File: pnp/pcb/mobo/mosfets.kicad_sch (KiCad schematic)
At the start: 0 parts

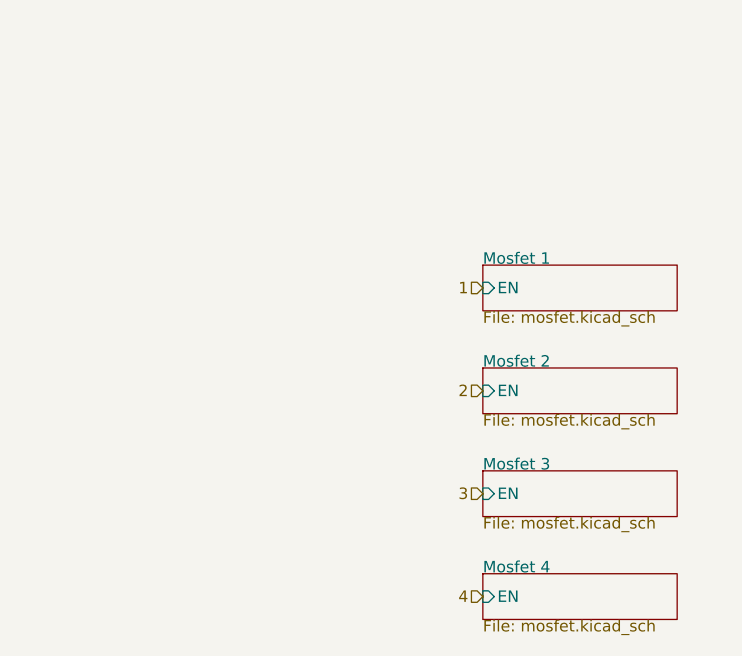
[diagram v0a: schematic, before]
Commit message: All pages checked
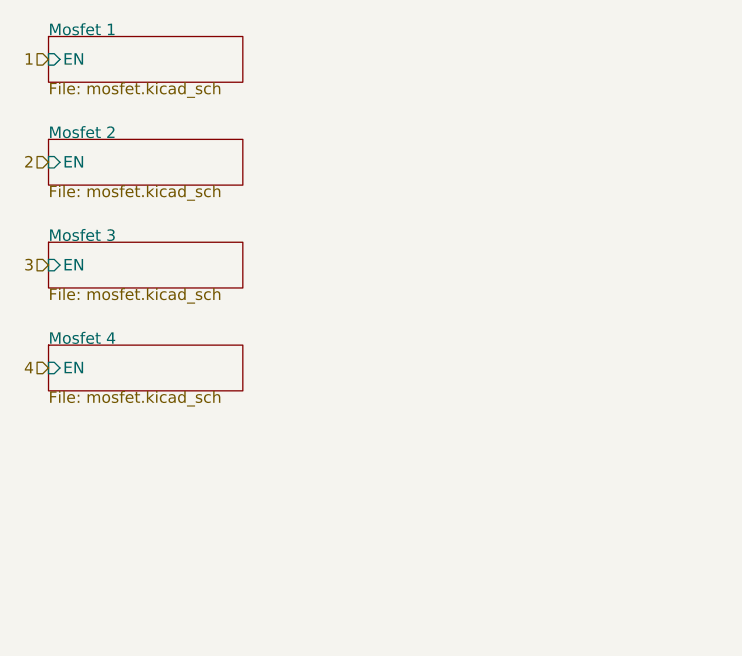
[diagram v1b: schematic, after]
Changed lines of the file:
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@@
 (kicad_sch (version 20230121) (generator eeschema)
-  (paper "A4")
+  (paper "A5")
   (title_block
     (title "LumenPnP Motherboard")
@@
     (rev "005")
     (company "Opulo")
+    (comment 1 "MOSFETs")
   )
-  (hierarchical_label "3" (shape input) (at 140.97 102.87 180) (fields_autoplaced)
+  (hierarchical_label "3" (shape input) (at 92.71 77.47 180) (fields_autoplaced)
     (effects (font (size 1.27 1.27)) (justify right))
   )
-  (hierarchical_label "2" (shape input) (at 140.97 91.44 180) (fields_autoplaced)
+  (hierarchical_label "2" (shape input) (at 92.71 66.04 180) (fields_autoplaced)
     (effects (font (size 1.27 1.27)) (justify right))
   )
-  (hierarchical_label "1" (shape input) (at 140.97 80.01 180) (fields_autoplaced)
+  (hierarchical_label "1" (shape input) (at 92.71 54.61 180) (fields_autoplaced)
     (effects (font (size 1.27 1.27)) (justify right))
   )
-  (hierarchical_label "4" (shape input) (at 140.97 114.3 180) (fields_autoplaced)
+  (hierarchical_label "4" (shape input) (at 92.71 88.9 180) (fields_autoplaced)
     (effects (font (size 1.27 1.27)) (justify right))
   )
-  (sheet (at 140.97 111.76) (size 21.59 5.08)
+  (sheet (at 92.71 86.36) (size 21.59 5.08)
     (stroke (width 0) (type solid))
     (fill (color 0 0 0 0.0000))
-    (property "Sheetname" "Mosfet 4" (at 140.97 111.76 0)
+    (property "Sheetname" "Mosfet 4" (at 92.71 86.36 0)
       (effects (font (size 1.27 1.27)) (justify left bottom))
     )
-    (property "Sheetfile" "mosfet.kicad_sch" (at 140.97 116.84 0)
+    (property "Sheetfile" "mosfet.kicad_sch" (at 92.71 91.44 0)
       (effects (font (size 1.27 1.27)) (justify left top))
     )
-    (pin "EN" input (at 140.97 114.3 180)
+    (pin "EN" input (at 92.71 88.9 180)
       (effects (font (size 1.27 1.27)) (justify left))
     )
@@
     )
   )
-  (sheet (at 140.97 88.9) (size 21.59 5.08)
+  (sheet (at 92.71 63.5) (size 21.59 5.08)
     (stroke (width 0) (type solid))
     (fill (color 0 0 0 0.0000))
-    (property "Sheetname" "Mosfet 2" (at 140.97 88.9 0)
+    (property "Sheetname" "Mosfet 2" (at 92.71 63.5 0)
       (effects (font (size 1.27 1.27)) (justify left bottom))
     )
-    (property "Sheetfile" "mosfet.kicad_sch" (at 140.97 93.98 0)
+    (property "Sheetfile" "mosfet.kicad_sch" (at 92.71 68.58 0)
       (effects (font (size 1.27 1.27)) (justify left top))
     )
-    (pin "EN" input (at 140.97 91.44 180)
+    (pin "EN" input (at 92.71 66.04 180)
       (effects (font (size 1.27 1.27)) (justify left))
     )
@@
     )
   )
-  (sheet (at 140.97 100.33) (size 21.59 5.08)
+  (sheet (at 92.71 74.93) (size 21.59 5.08)
     (stroke (width 0) (type solid))
     (fill (color 0 0 0 0.0000))
-    (property "Sheetname" "Mosfet 3" (at 140.97 100.33 0)
+    (property "Sheetname" "Mosfet 3" (at 92.71 74.93 0)
       (effects (font (size 1.27 1.27)) (justify left bottom))
     )
-    (property "Sheetfile" "mosfet.kicad_sch" (at 140.97 105.41 0)
+    (property "Sheetfile" "mosfet.kicad_sch" (at 92.71 80.01 0)
       (effects (font (size 1.27 1.27)) (justify left top))
     )
-    (pin "EN" input (at 140.97 102.87 180)
+    (pin "EN" input (at 92.71 77.47 180)
       (effects (font (size 1.27 1.27)) (justify left))
     )
@@
     )
   )
-  (sheet (at 140.97 77.47) (size 21.59 5.08)
+  (sheet (at 92.71 52.07) (size 21.59 5.08)
     (stroke (width 0) (type solid))
     (fill (color 0 0 0 0.0000))
-    (property "Sheetname" "Mosfet 1" (at 140.97 77.47 0)
+    (property "Sheetname" "Mosfet 1" (at 92.71 52.07 0)
       (effects (font (size 1.27 1.27)) (justify left bottom))
     )
-    (property "Sheetfile" "mosfet.kicad_sch" (at 140.97 82.55 0)
+    (property "Sheetfile" "mosfet.kicad_sch" (at 92.71 57.15 0)
       (effects (font (size 1.27 1.27)) (justify left top))
     )
-    (pin "EN" input (at 140.97 80.01 180)
+    (pin "EN" input (at 92.71 54.61 180)
       (effects (font (size 1.27 1.27)) (justify left))
     )
